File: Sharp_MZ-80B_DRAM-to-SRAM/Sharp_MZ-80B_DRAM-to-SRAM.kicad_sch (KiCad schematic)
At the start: 6 parts, among them CN1 RAM III & IV, U1 CY62256-70PC, U2 CY62256-70PC, U35 74LS244, U36 74LS244, U37 74LS04

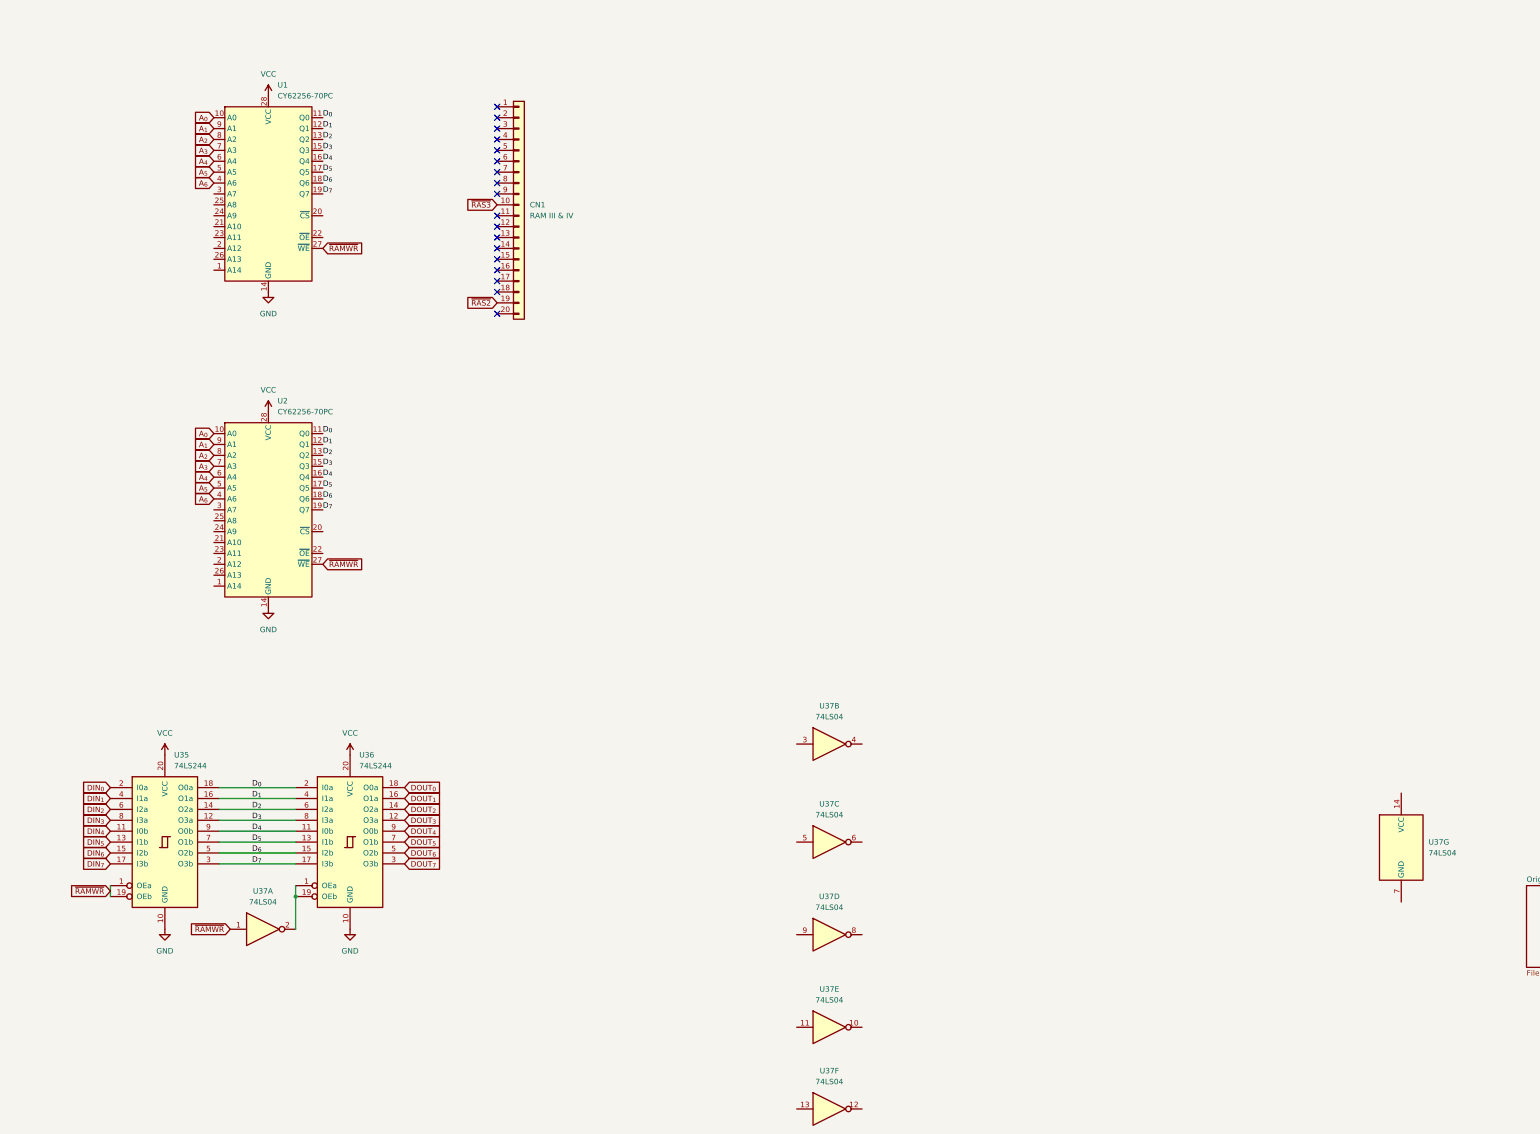
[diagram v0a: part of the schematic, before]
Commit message: Initial design completed
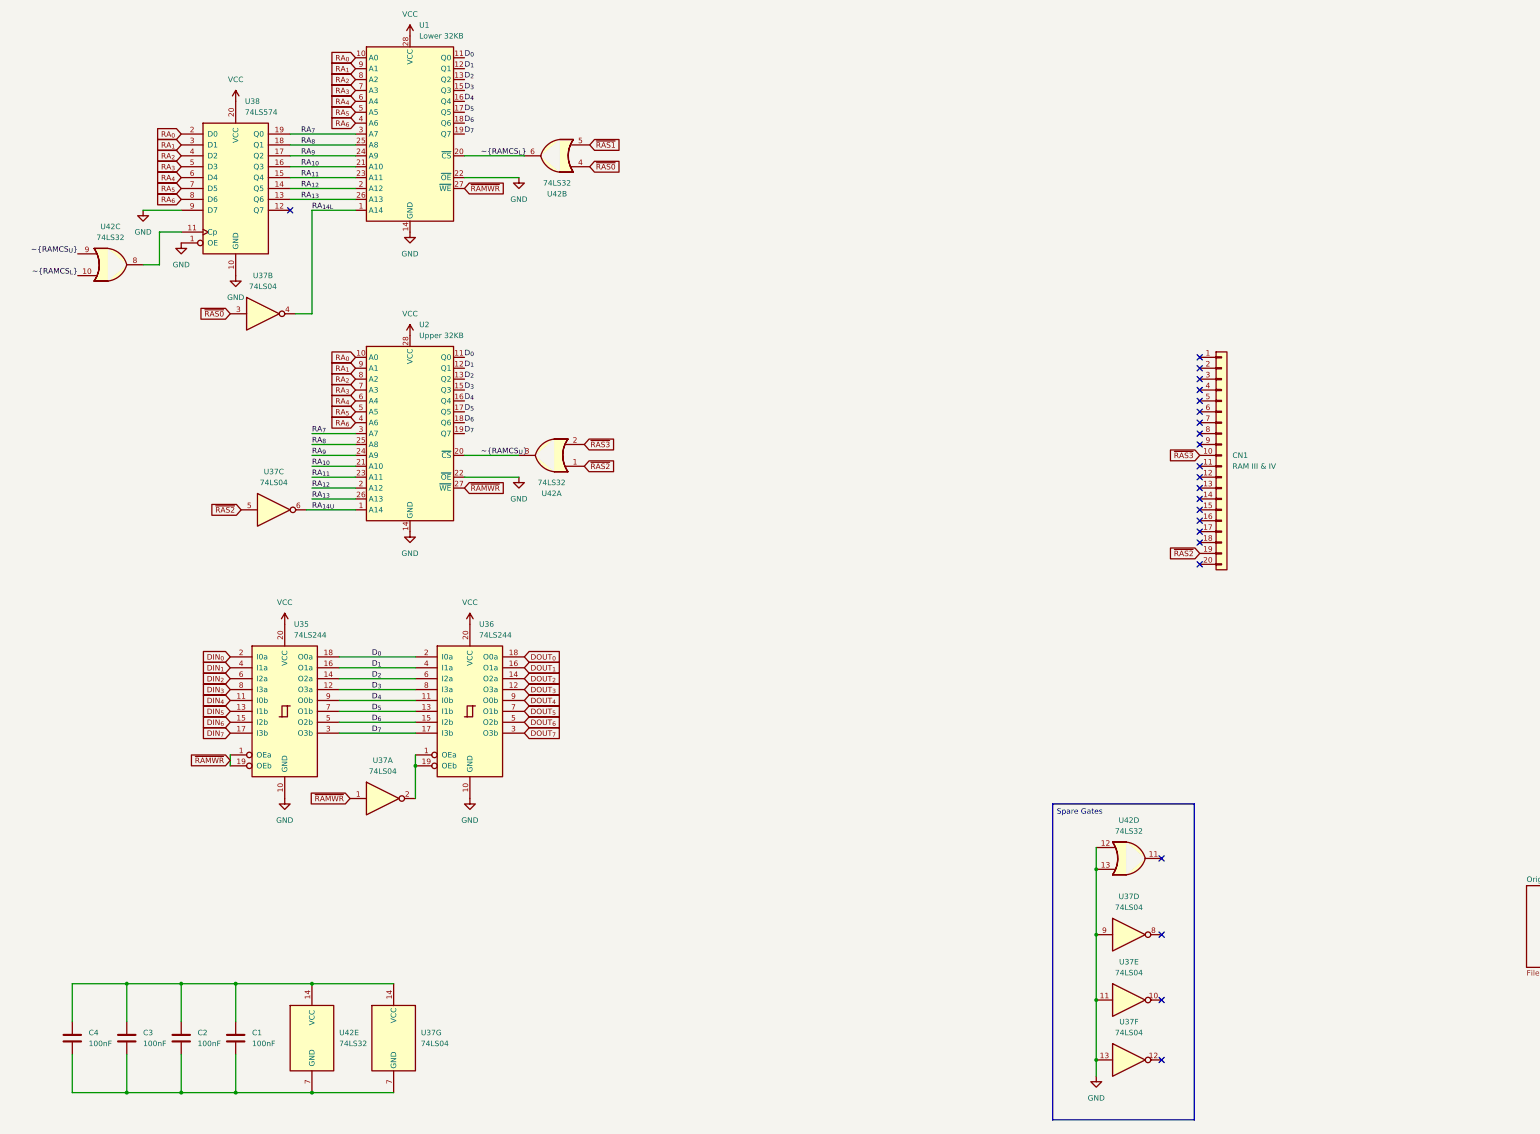
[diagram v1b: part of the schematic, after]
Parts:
- added C1, C2, C3, C4: 100nF, symbol Device:C
- added U38: 74LS574, symbol 74xx:74LS574
- added U42: 74LS32, symbol 74xx:74LS32
- U1: value CY62256-70PC -> Lower 32KB
- U2: value CY62256-70PC -> Upper 32KB
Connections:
- net GND: now also U1.22 (~{OE}), U2.22 (~{OE}), U37.11, U37.13, U37.9, U38.1 (OE), U38.10 (GND), U38.9 (D7), U42.12, U42.13
- net VCC: now also U38.20 (VCC)
- net ~{RAS2}: now also U37.5, U42.1
- net ~{RAS3}: now also U42.2
- net RA_{14U}: now reaches U2.1 (A14)
- net RA_{14U}: now also U37.6
- net RA_{12}: now reaches U2.2 (A12)
- net RA_{12}: now also U1.2 (A12), U38.14 (Q5)
- net ~{RAMCS_{U}}: now reaches U2.20 (~{CS})
- net ~{RAMCS_{U}}: now also U42.3, U42.9
- net RA_{10}: now reaches U2.21 (A10)
- net RA_{10}: now also U1.21 (A10), U38.16 (Q3)
- net RA_{11}: now reaches U2.23 (A11)
- net RA_{11}: now also U1.23 (A11), U38.15 (Q4)
- net RA_{9}: now reaches U2.24 (A9)
- net RA_{9}: now also U1.24 (A9), U38.17 (Q2)
- net RA_{8}: now reaches U2.25 (A8)
- net RA_{8}: now also U1.25 (A8), U38.18 (Q1)
- net RA_{13}: now reaches U2.26 (A13)
- net RA_{13}: now also U1.26 (A13), U38.13 (Q6)
- net RA_{7}: now reaches U2.3 (A7)
- net RA_{7}: now also U1.3 (A7), U38.19 (Q0)
- net RA_{14L}: now reaches U1.1 (A14)
- net RA_{14L}: now also U37.4
- net ~{RAMCS_{L}}: now reaches U1.20 (~{CS})
- net ~{RAMCS_{L}}: now also U42.10, U42.6
- net at U37.14 (VCC): now also C1.1, C2.1, C3.1, C4.1, U42.14 (VCC)
- net at U37.7 (GND): now also C1.2, C2.2, C3.2, C4.2, U42.7 (GND)
- net ~{RAS0}: now reaches U37.3
- net ~{RAS0}: now also U42.4
- net A_{0} renamed RA_{0}
- net RA_{0}: now also U38.2 (D0)
- net A_{1} renamed RA_{1}
- net RA_{1}: now also U38.3 (D1)
- net A_{2} renamed RA_{2}
- net RA_{2}: now also U38.4 (D2)
- net A_{3} renamed RA_{3}
- net RA_{3}: now also U38.5 (D3)
- net A_{4} renamed RA_{4}
- net RA_{4}: now also U38.6 (D4)
- net A_{5} renamed RA_{5}
- net RA_{5}: now also U38.7 (D5)
- net A_{6} renamed RA_{6}
- net RA_{6}: now also U38.8 (D6)
- new net: U38.11 (Cp), U42.8
- new net ~{RAS1}: U42.5
- no-connect marks 18 -> 23
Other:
- company: (none) -> Brett Hallen
- title: (none) -> Sharp MZ-80B SRAM Replacement
- moved on the sheet: CN1, U1, U2, U35, U36, U37A, U37B, U37C, U37D, U37E, U37F, U37G
